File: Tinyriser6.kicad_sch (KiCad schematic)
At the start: 24 parts, among them J1 Bus_M.2_Socket_M, J10 Conn_02x04_Odd_Even, J11 Conn_02x04_Odd_Even, J2 Bus_PCI_Express_x16, J3 Conn_02x04_Odd_Even, J6 USB_A, J8 Conn_02x04_Odd_Even, J9 Conn_02x04_Odd_Even, M1 Fan_4pin

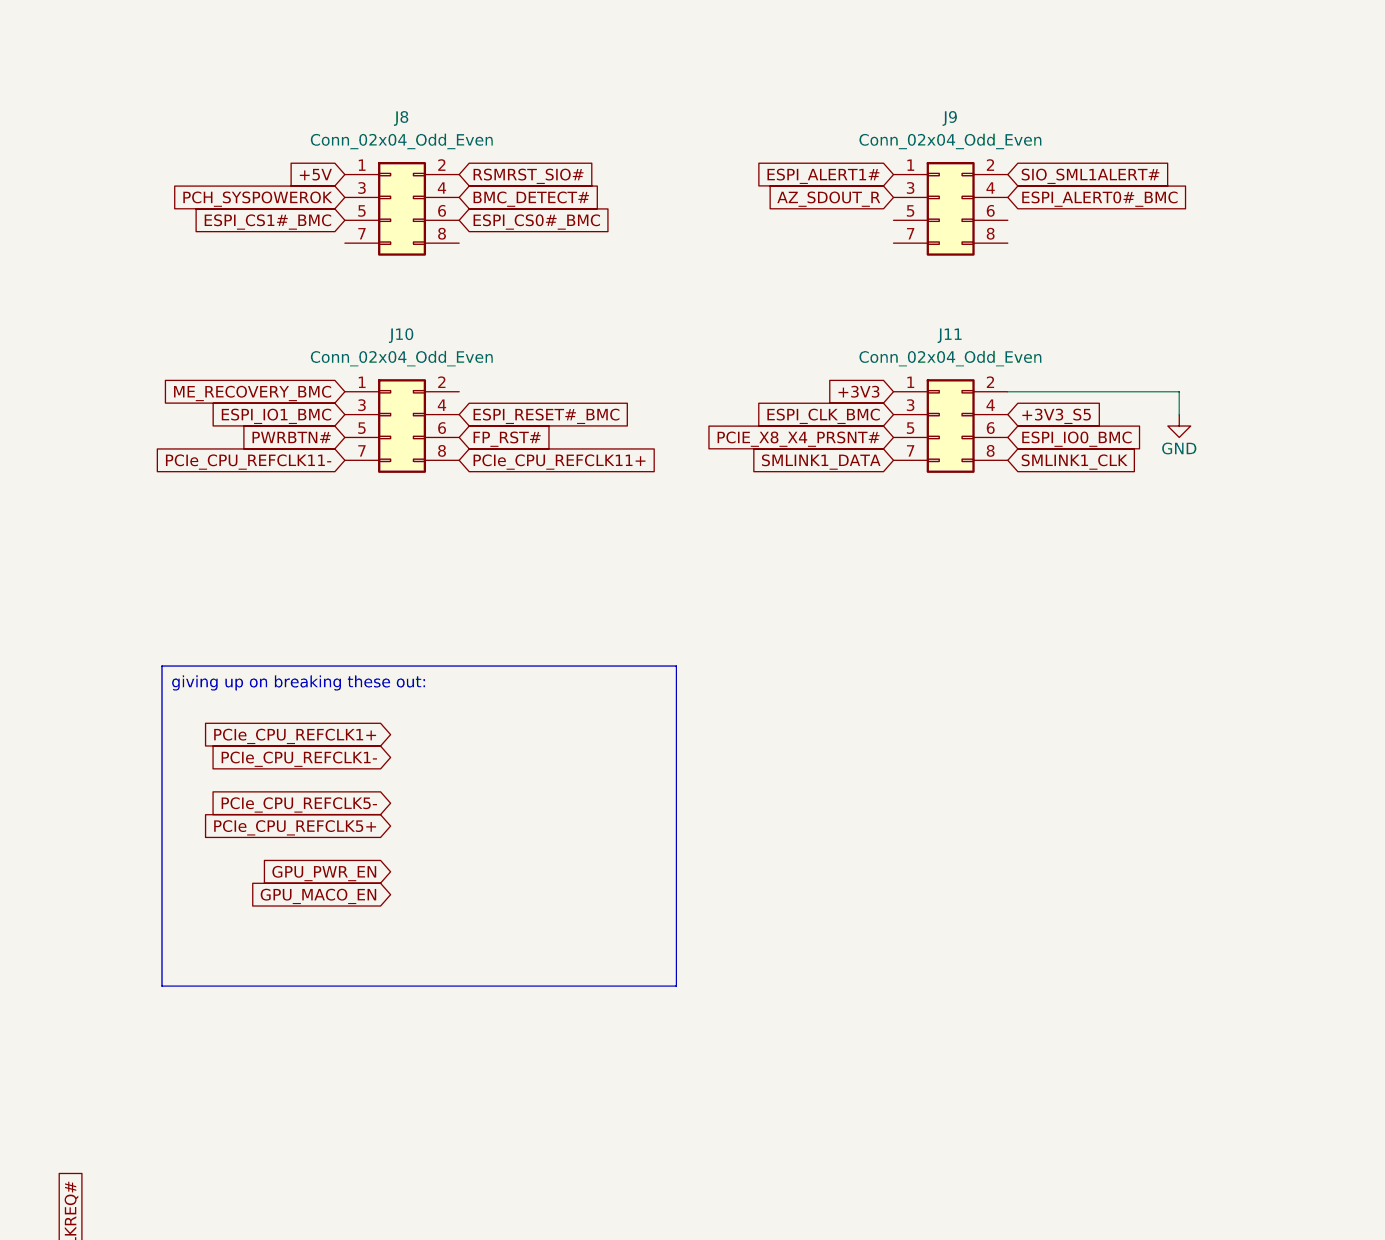
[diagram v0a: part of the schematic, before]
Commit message: giving up on breaking out ESPI, tuned some diffpairs
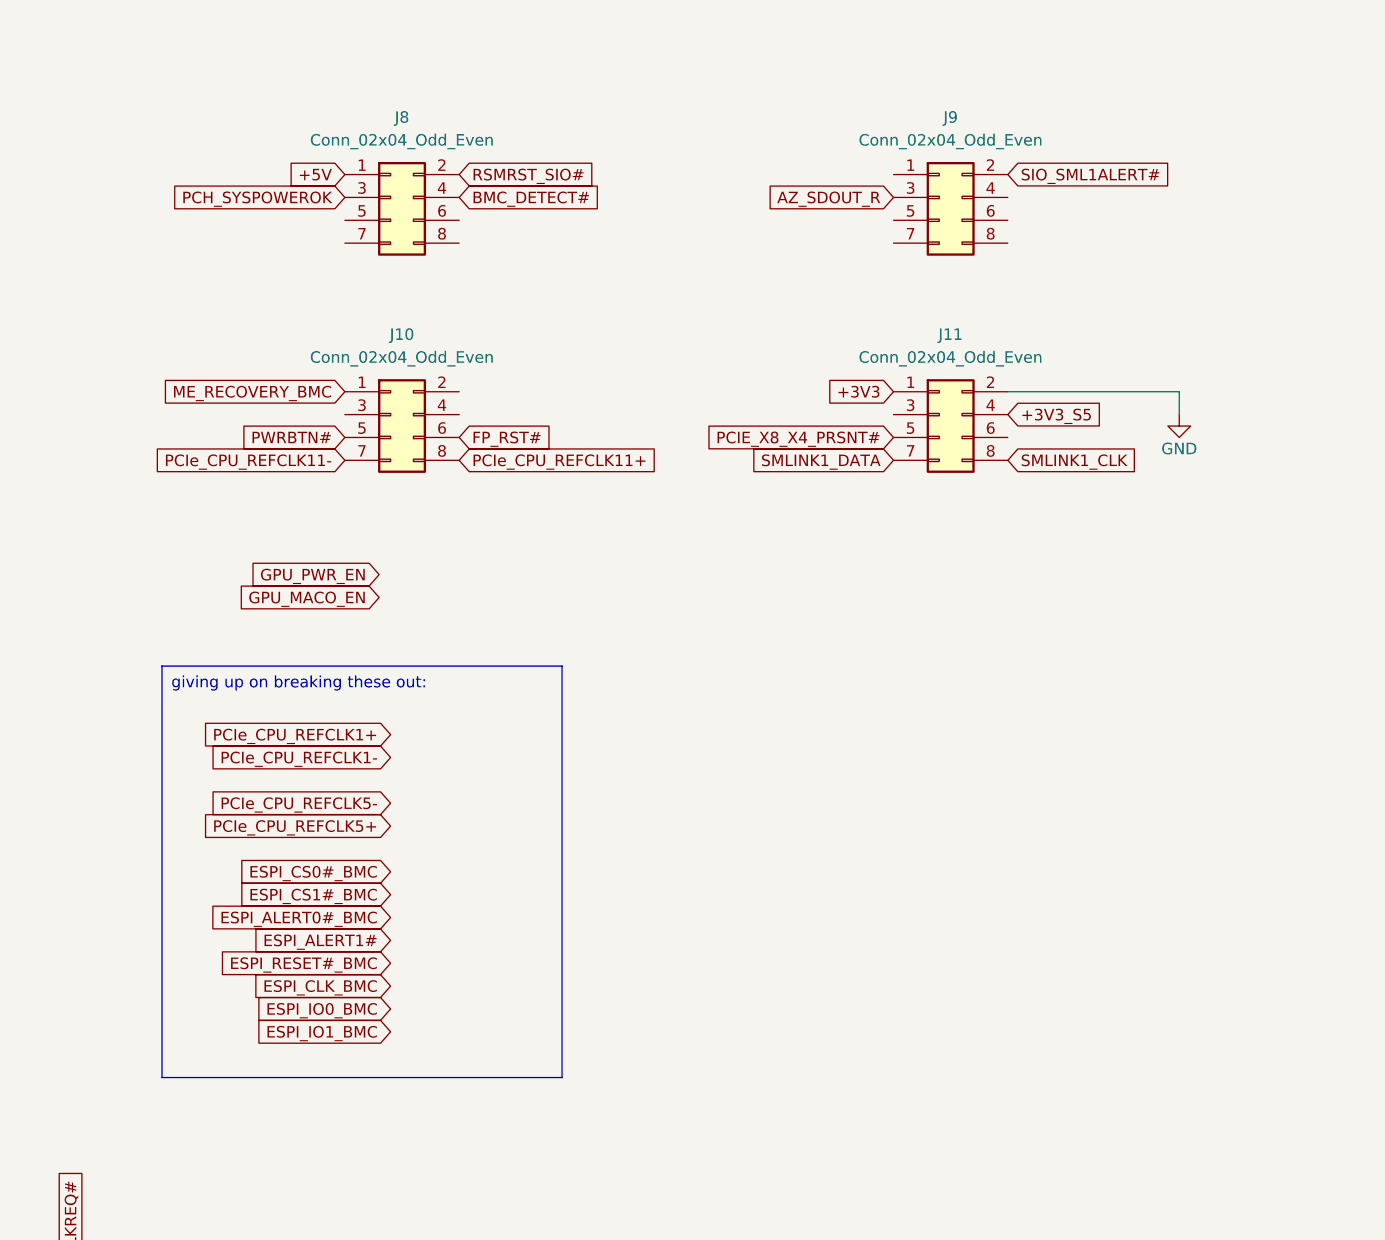
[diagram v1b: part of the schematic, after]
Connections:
- net ESPI_ALERT0#_BMC: no longer J9.4 (Pin_4)
- net ESPI_ALERT1#: no longer J9.1 (Pin_1)
- net ESPI_CLK_BMC: no longer J11.3 (Pin_3)
- net ESPI_CS0#_BMC: no longer J8.6 (Pin_6)
- net ESPI_CS1#_BMC: no longer J8.5 (Pin_5)
- net ESPI_IO0_BMC: no longer J11.6 (Pin_6)
- net ESPI_IO1_BMC: no longer J10.3 (Pin_3)
- net ESPI_RESET#_BMC: no longer J10.4 (Pin_4)
